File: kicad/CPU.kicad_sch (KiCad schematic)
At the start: 37 parts, among them J1 Conn_ARM_SWD_TagConnect_TC203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, J2 Screw_Terminal_01x03, J3 Screw_Terminal_01x03, SW1 SW_Push, U7 STM32F303CBTx, Y1 8 MHz

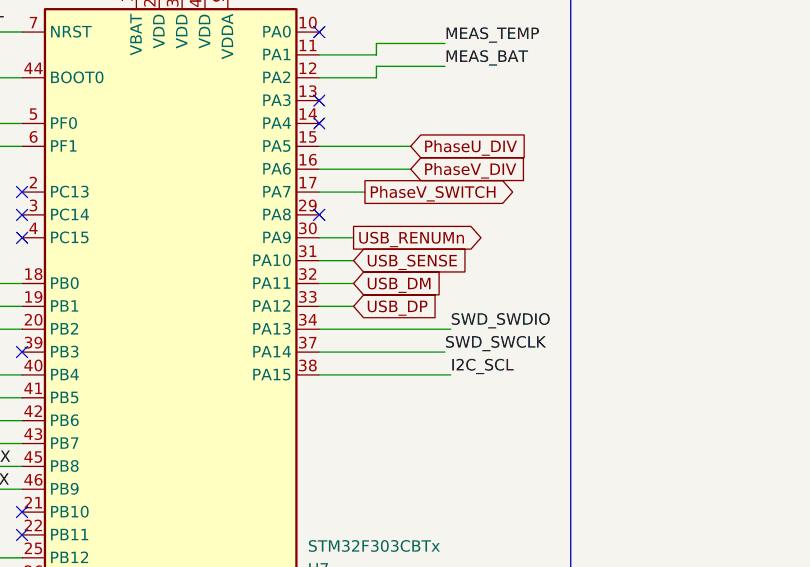
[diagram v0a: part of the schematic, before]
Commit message: [kicad] Layout, mostly power traces + HS signal traces
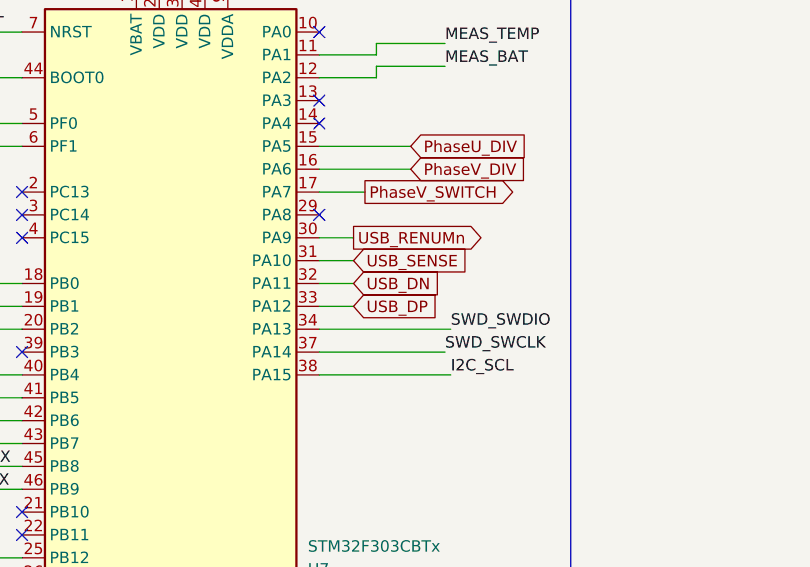
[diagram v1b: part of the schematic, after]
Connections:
- net USB_DM renamed USB_DN
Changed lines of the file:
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@@
     )
   )
-  (global_label "USB_DM" (shape input) (at 118.11 140.97 0) (fields_autoplaced)
+  (global_label "USB_DN" (shape input) (at 118.11 140.97 0) (fields_autoplaced)
     (effects (font (size 1.27 1.27)) (justify left))
-    (property "Intersheetrefs" "${INTERSHEET_REFS}" (at 128.5942 140.97 0)
+    (property "Intersheetrefs" "${INTERSHEET_REFS}" (at 128.4733 140.97 0)
       (effects (font (size 1.27 1.27)) (justify left) hide)
     )
